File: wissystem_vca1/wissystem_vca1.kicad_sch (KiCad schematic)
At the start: 15 parts, among them J1 EuroPower16, U1 TL072CDT, U2 XL13700

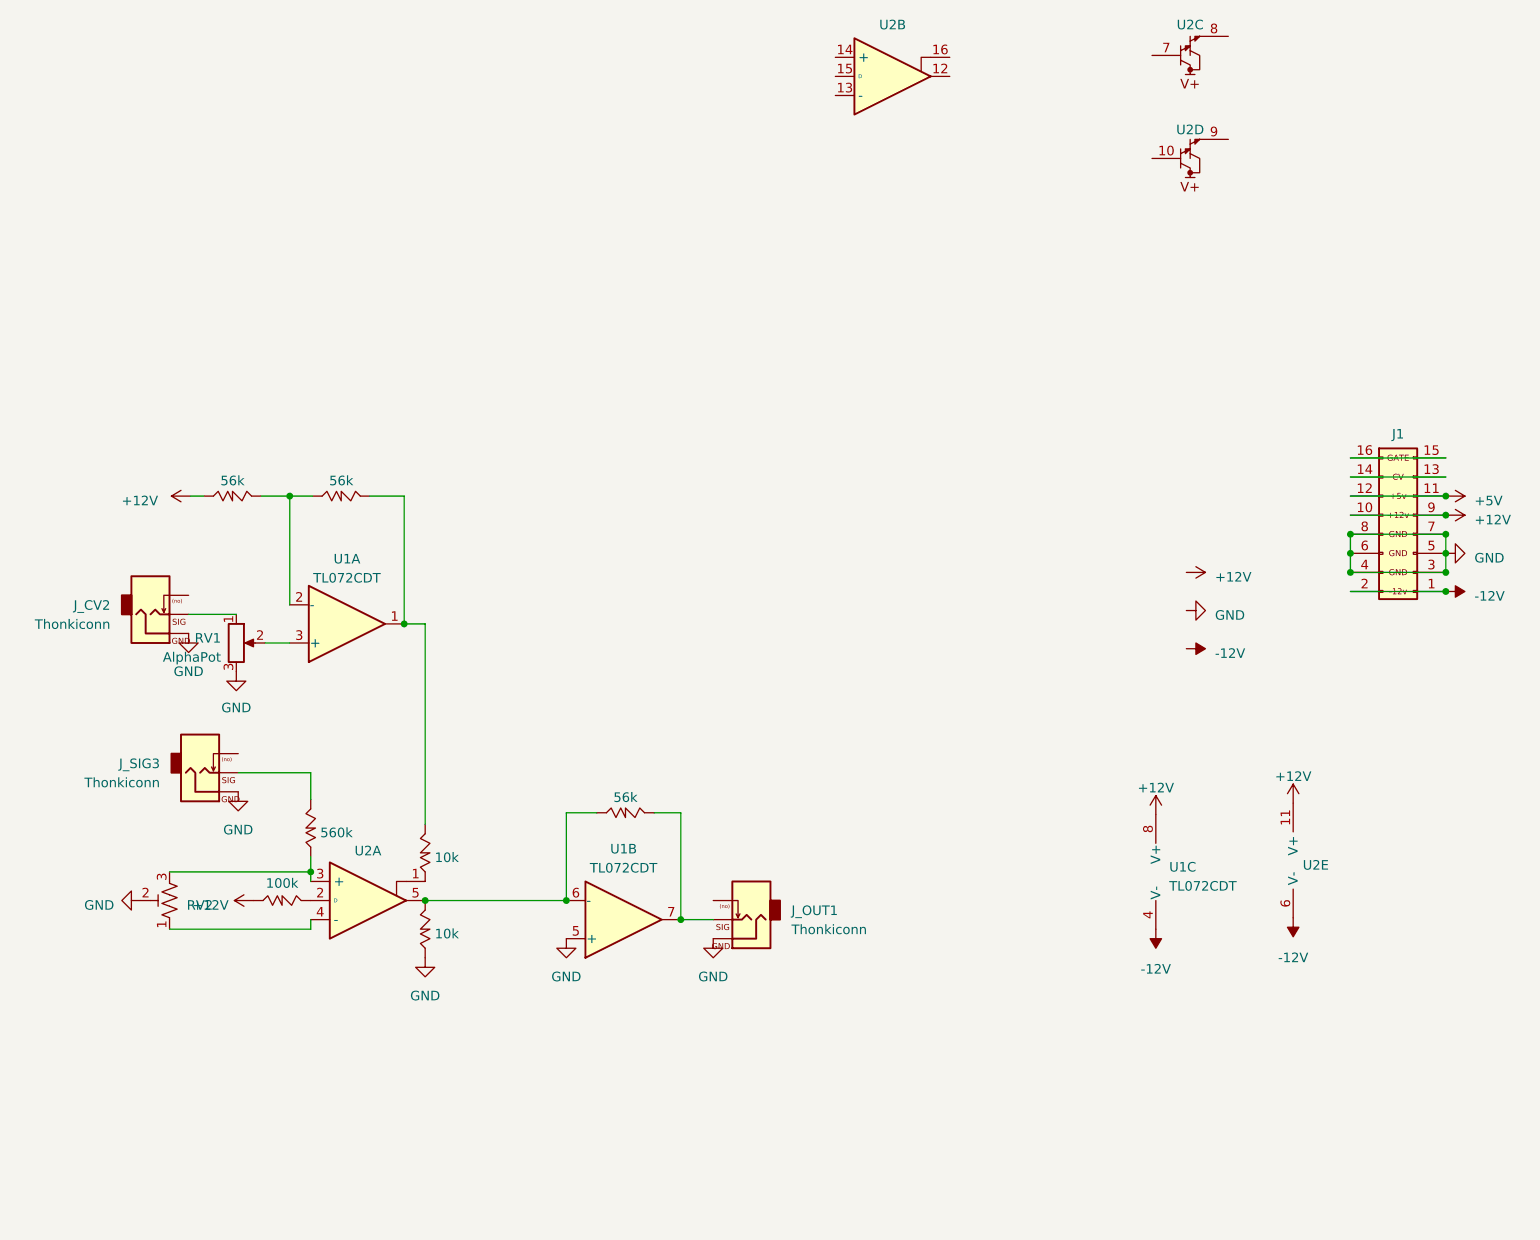
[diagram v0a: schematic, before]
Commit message: asdf
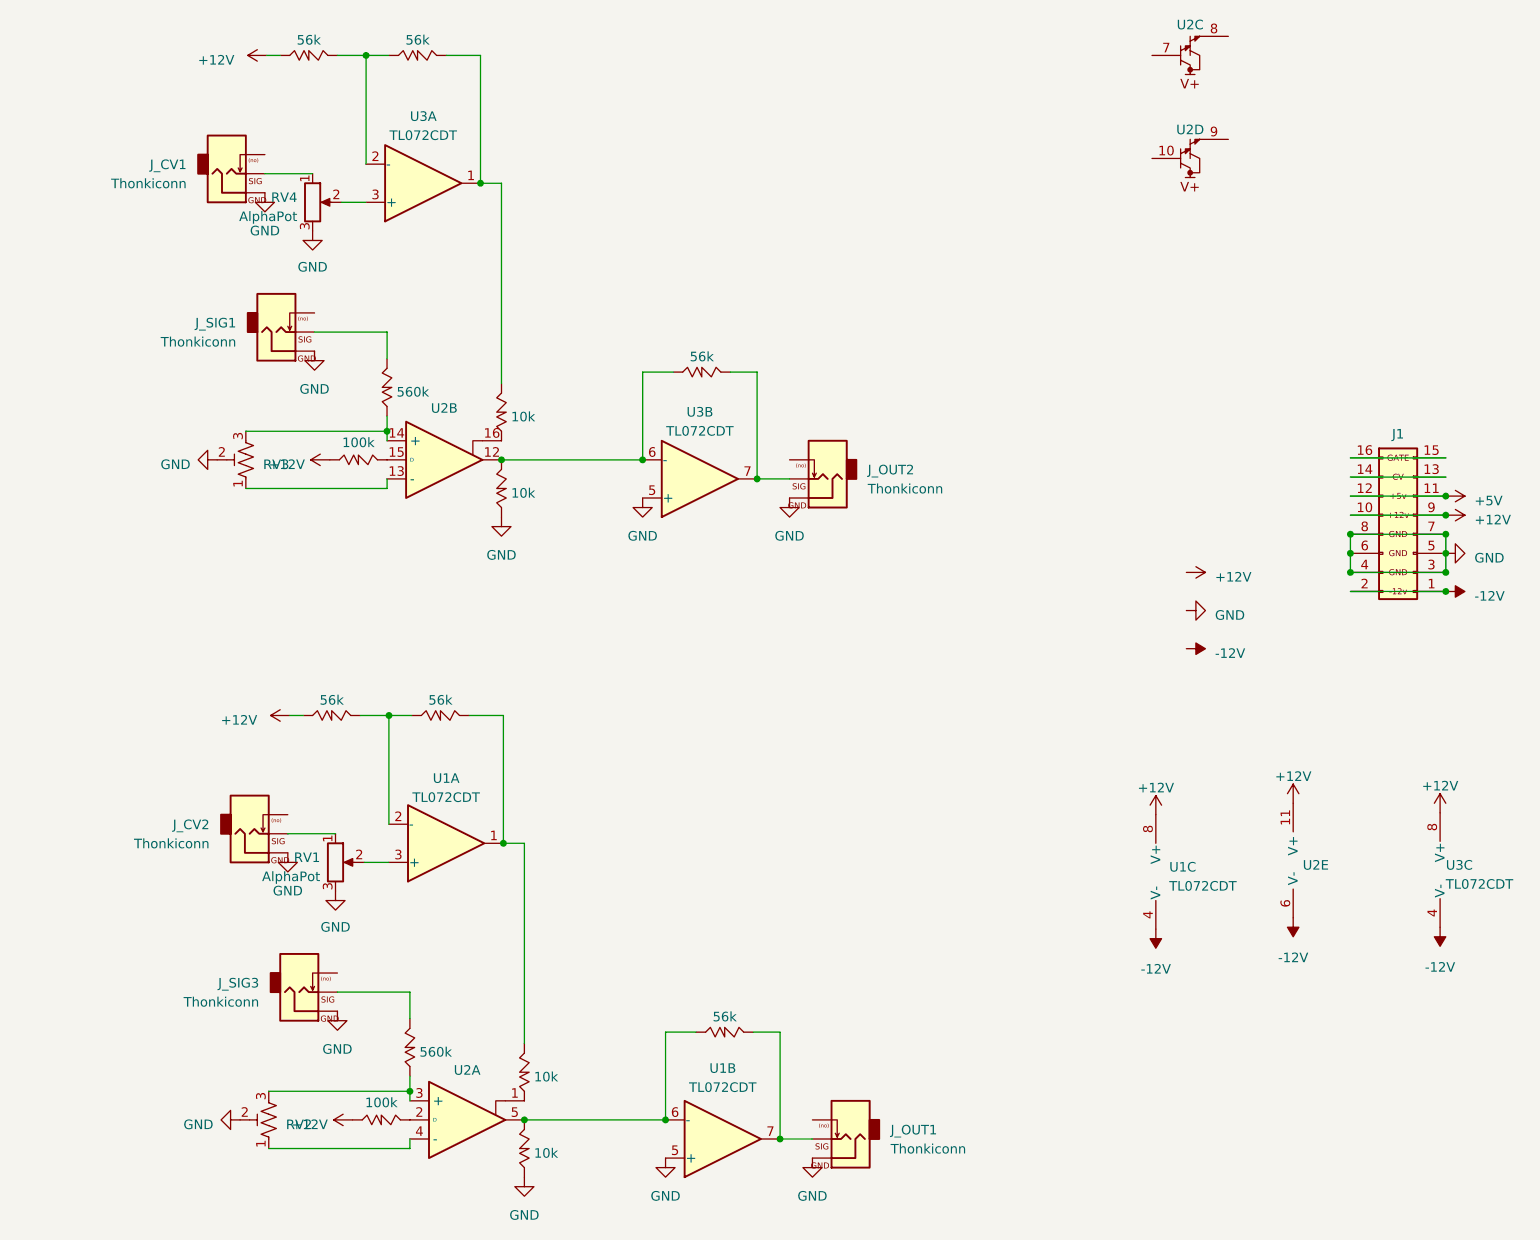
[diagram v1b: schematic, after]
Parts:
- added J_CV1, J_OUT2, J_SIG1: Thonkiconn, Connector_Audio:Jack_3.5mm_QingPu_WQP-PJ398SM_Vertical_CircularHoles, symbol EuroRackTools:Thonkiconn
- added R10: 560k, kpm-jlcpcb-basic:R_0603_1608Metric, symbol kpm-jlcpcb-basic:560k R 0603
- added R11, R14, R8: 56k, kpm-jlcpcb-basic:R_0402_1005Metric, symbol kpm-jlcpcb-basic:56k R 0402
- added R12, R13: 10k, kpm-jlcpcb-basic:R_0402_1005Metric, symbol kpm-jlcpcb-basic:10k R 0402
- added R9: 100k, kpm-jlcpcb-basic:R_0402_1005Metric, symbol kpm-jlcpcb-basic:100k R 0402
- added RV3: R_Potentiometer_Trim_US, Potentiometer_SMD:Potentiometer_Bourns_TC33X_Vertical, symbol EuroRackTools:TRIMPOT
- added RV4: AlphaPot, Potentiometer_THT:Potentiometer_Alpha_RD901F-40-00D_Single_Vertical, symbol EuroRackTools:AlphaPot
- added U3: TL072CDT, kpm-jlcpcb-basic:SOIC-8_3.9x4.9mm_P1.27mm, symbol kpm-jlcpcb-basic:TL072CDT
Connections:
- net +12V: now also R8.1, R9.1, U3.8 (V+)
- net -12V: now also U3.4 (V-)
- net GND: now also J_CV1.S, J_OUT2.S, J_SIG1.S, R13.1, RV3.2, RV4.3, U3.5 (+)
- net at U2.12: now also R13.2, R14.1, U3.6 (-)
- net at U2.13 (-): now also RV3.1
- net at U2.14 (+): now also R10.1, RV3.3
- net at U2.15 (D): now also R9.2
- net at U2.16: now also R12.1
- new net: J_OUT2.T, R14.2, U3.7
- new net: J_SIG1.T, R10.2
- new net: J_CV1.T, RV4.1
- new net: R11.2, R12.2, U3.1
- new net: R11.1, R8.2, U3.2 (-)
- new net: RV4.2, U3.3 (+)
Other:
- moved on the sheet: J_CV2, J_OUT1, J_SIG3, RV1, RV2, U1A, U1B, U2A, U2B
